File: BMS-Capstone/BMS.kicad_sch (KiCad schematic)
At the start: 0 parts

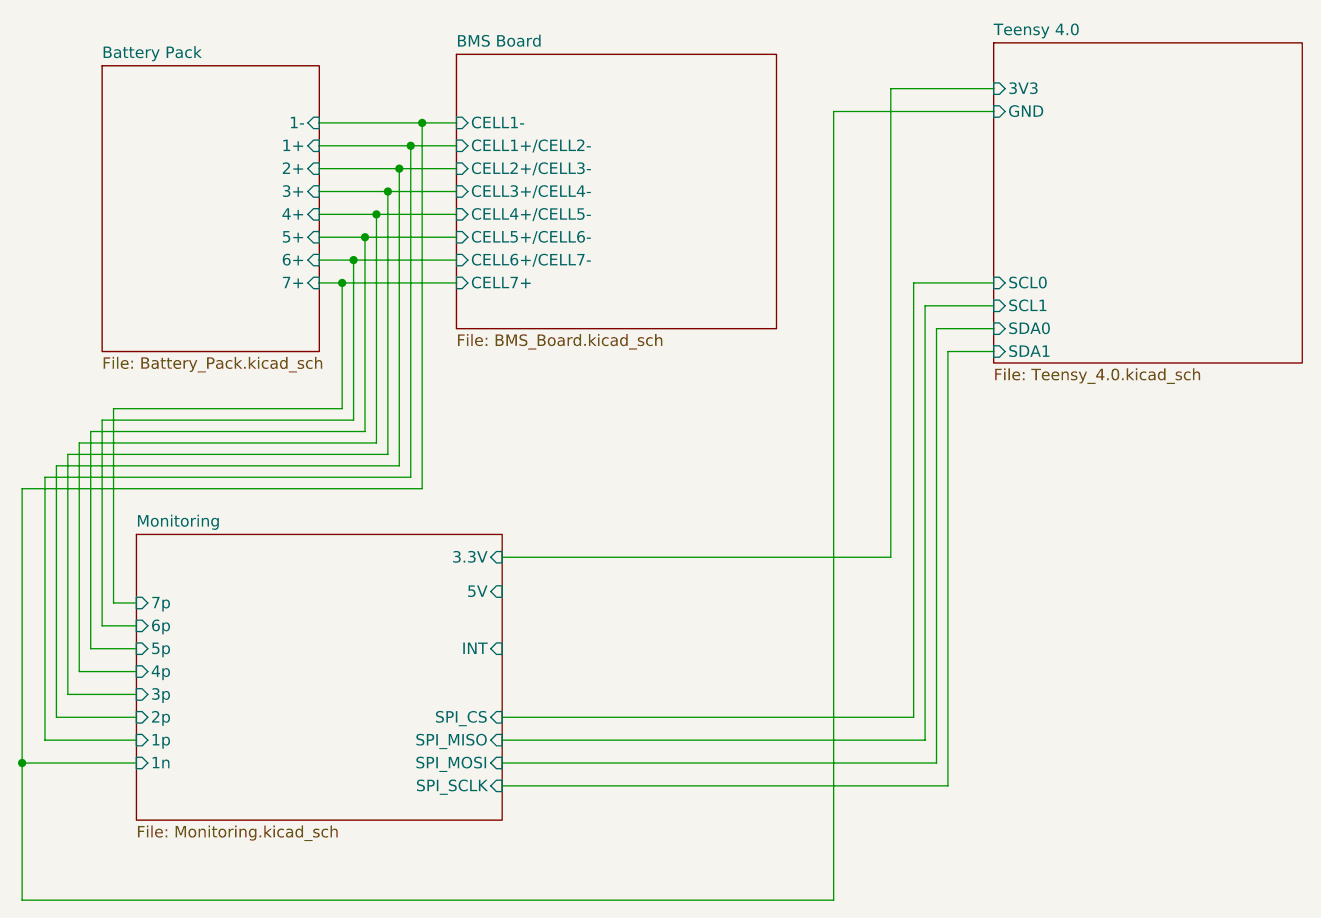
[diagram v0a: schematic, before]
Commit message: routing for TI chip
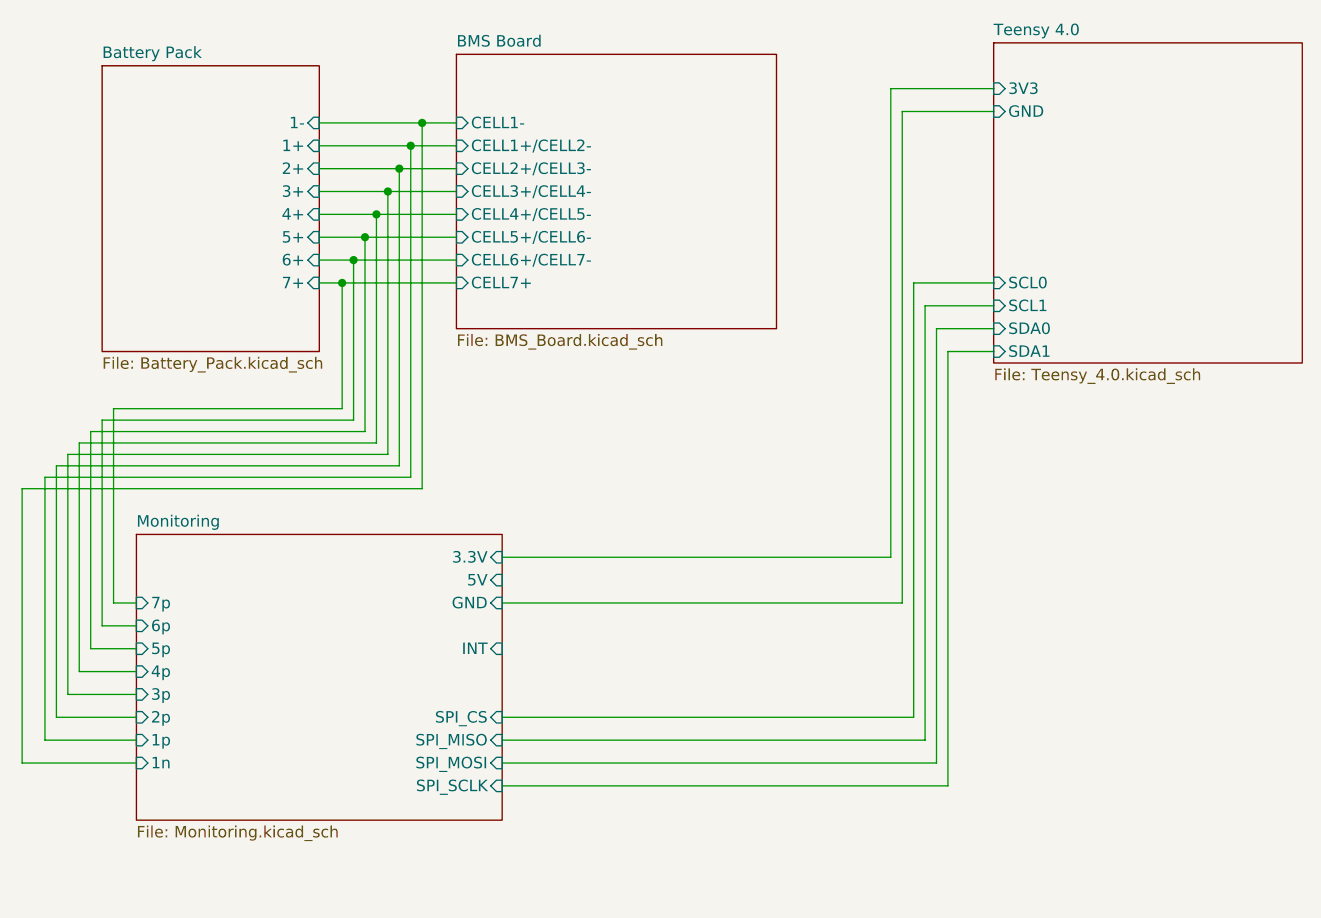
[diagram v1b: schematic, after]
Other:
- sheet Monitoring ports: added GND; removed none
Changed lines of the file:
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@@
-	)
-	(junction
-		(at 53.34 124.46)
-		(diameter 0)
-		(color 0 0 0 0)
 	)
 	(junction
@@
 	(wire
 		(pts
-			(xy 143.51 52.07) (xy 143.51 139.7)
-		)
-		(stroke
-			(width 0)
-			(type default)
-		)
-	)
-	(wire
-		(pts
 			(xy 156.21 78.74) (xy 161.29 78.74)
 		)
@@
 	(wire
 		(pts
-			(xy 143.51 139.7) (xy 53.34 139.7)
-		)
-		(stroke
-			(width 0)
-			(type default)
-		)
-	)
-	(wire
-		(pts
 			(xy 106.68 119.38) (xy 152.4 119.38)
 		)
@@
 	(wire
 		(pts
+			(xy 161.29 52.07) (xy 151.13 52.07)
+		)
+		(stroke
+			(width 0)
+			(type default)
+		)
+	)
+	(wire
+		(pts
 			(xy 96.52 55.88) (xy 101.6 55.88)
 		)
@@
 	(wire
 		(pts
-			(xy 53.34 139.7) (xy 53.34 124.46)
-		)
-		(stroke
-			(width 0)
-			(type default)
-		)
-	)
-	(wire
-		(pts
 			(xy 66.04 121.92) (xy 55.88 121.92)
 		)
@@
 	(wire
 		(pts
+			(xy 151.13 106.68) (xy 106.68 106.68)
+		)
+		(stroke
+			(width 0)
+			(type default)
+		)
+	)
+	(wire
+		(pts
 			(xy 59.69 114.3) (xy 59.69 88.9)
 		)
@@
 	(wire
 		(pts
-			(xy 161.29 52.07) (xy 143.51 52.07)
-		)
-		(stroke
-			(width 0)
-			(type default)
-		)
-	)
-	(wire
-		(pts
 			(xy 58.42 116.84) (xy 58.42 90.17)
 		)
@@
 		(pts
 			(xy 106.68 101.6) (xy 149.86 101.6)
+		)
+		(stroke
+			(width 0)
+			(type default)
+		)
+	)
+	(wire
+		(pts
+			(xy 151.13 52.07) (xy 151.13 106.68)
 		)
 		(stroke
@@
 		)
 		(pin "5V" input
-			(at 106.68 105.41 0)
+			(at 106.68 104.14 0)
 			(effects
 				(font
@@
 			(effects
 				(font
+					(size 1.27 1.27)
+				)
+				(justify right)
+			)
+		)
+		(pin "GND" input
+			(at 106.68 106.68 0)
+			(effects
+				(font
